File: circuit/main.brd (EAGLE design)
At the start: 21.6 x 21.3 mm, 18 parts, among them IC2 LD398533RM, J1 22-27-2041-04, J2 22-27-2041-04, Q2 BSS138, Q3 12MHz, U1 ATTINY84-20SSU

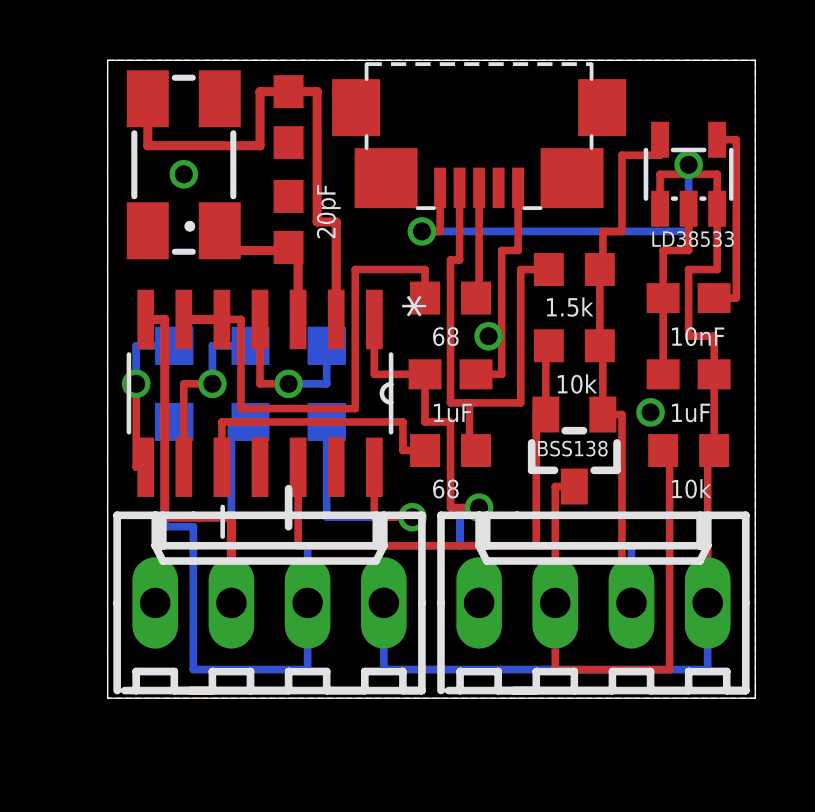
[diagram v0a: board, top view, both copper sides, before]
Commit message: my own board
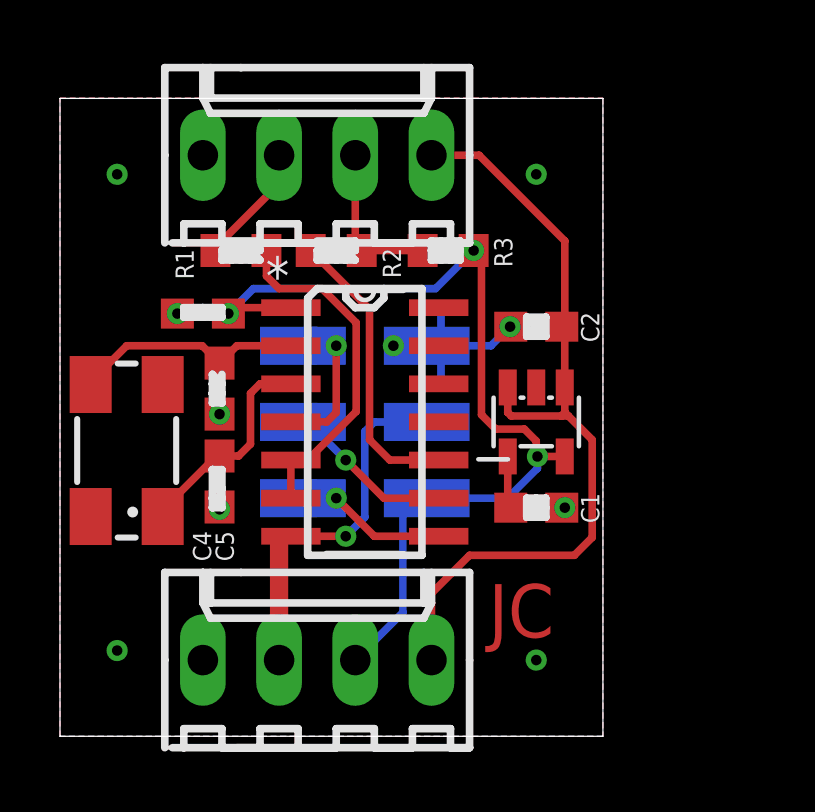
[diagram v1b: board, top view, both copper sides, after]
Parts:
- removed J2: 22-27-2041-04, con-molex:6410-04
- removed Q2: BSS138, m-pad-2.1:SOT23
- removed R4, R5: 10k, resistor:R0603
- removed U$3: MICRO-USB-ZX62R-B-5P, con-hirose:ZX62R-B-5P
- added J4: 22-27-2041-04, con-molex:6410-04
- R1, R2: value 68 -> 100r
- moved Q3 9.71 mm to (2.22, 9.53)
- moved IC2 9.69 mm to (15.9, 10.5), turned to 180 degrees
- moved C4 9.34 mm to (5.32, 11.6)
- moved C5 8.95 mm to (5.32, 8.49), turned to 90 degrees
- moved C1 8.64 mm to (15.9, 7.62), turned to 0 degrees
- moved C3 8.50 mm to (4.76, 14.1), turned to 0 degrees
- moved R2 7.68 mm to (9.21, 16.2)
- moved R1 7.16 mm to (6.03, 16.2), turned to 180 degrees
- moved C2 5.32 mm to (15.9, 13.7)
- moved R3 4.25 mm to (12.9, 16.2)
- moved U1 3.62 mm to (10.2, 10.5), turned to 0 degrees
- moved U$1 3.59 mm to (11.4, 13.0), turned to 180 degrees
- moved J1 2.48 mm to (8.57, 2.54)
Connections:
- removed net ID: U$3.4
- removed net N$1: Q2.2, R4.1, U1.12
- removed net SIG2: J2.3, Q2.3, R5.1
- net 3.3V: no longer J2.2, Q2.1, R4.2
- net 5V: now also J4.1; no longer J2.1, R5.2, U$3.1
- net GND: now also J4.4; no longer J2.4, U$3.5
- net N$2: now also J4.2; no longer U$3.2
- net N$5: now also J4.3; no longer U$3.3
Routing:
- net 3.3V: track 61.0 -> 31.8 mm, vias 1 -> 3
- net 5V: track 48.1 -> 27.8 mm, vias 2 -> 0
- net SIG2: track 18.6 -> 0.00 mm
- net N$1: track 17.6 -> 0.00 mm
- net GND: track 23.0 -> 6.16 mm, vias 4 -> 10
- net N$2: track 17.0 -> 5.29 mm
- net XTAL1: track 17.2 -> 7.81 mm
- net MOSI/SIG1: track 19.0 -> 11.5 mm, vias 0 -> 1
- net USB_D+: track 16.6 -> 11.6 mm
- net N$4: track 6.65 -> 1.75 mm
- net XTAL2: track 5.31 -> 7.23 mm
- net RESET: track 5.64 -> 3.87 mm
- net MISO: track 5.64 -> 3.94 mm
- net USCK: track 6.27 -> 5.16 mm
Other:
- board size 21.6 x 21.3 mm -> 18.1 x 21.3 mm
- board text added: "+5v"
- board text added: "D+"
- board text added: "D-"
- board text added: "GCD"
- board text added: "JC"
- board text removed: "BSS138"
- board text removed: "Garrett Greenwood"
- board text removed: "LD38533"
- board text removed: "SIG1"
- board text removed: "SIG2"
- board text removed: "Shinewave v0.3.1"
